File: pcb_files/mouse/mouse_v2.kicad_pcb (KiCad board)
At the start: 2 copper layers, 94.7 x 94.9 mm, 72 parts, among them J2 BT_Conn, J4 I2C_Conn, M1 Motor_DC, M2 Motor_DC, M3 CASTER_BALL, Q0 Q_Photo_NPN, Q1 Q_Photo_NPN, Q2 Q_Photo_NPN, Q3 Q_Photo_NPN, SW1 TL3315NF160Q, SW2 TL3315NF160Q, T0 Q_NMOS_DGS, T1 Q_NMOS_DGS, T2 Q_NMOS_DGS, T3 Q_NMOS_DGS, U1 Teensy3.2, U2 SN754410NE, U3 LM1084-5.0, U4 Encoder_3081, U5 Encoder_3081

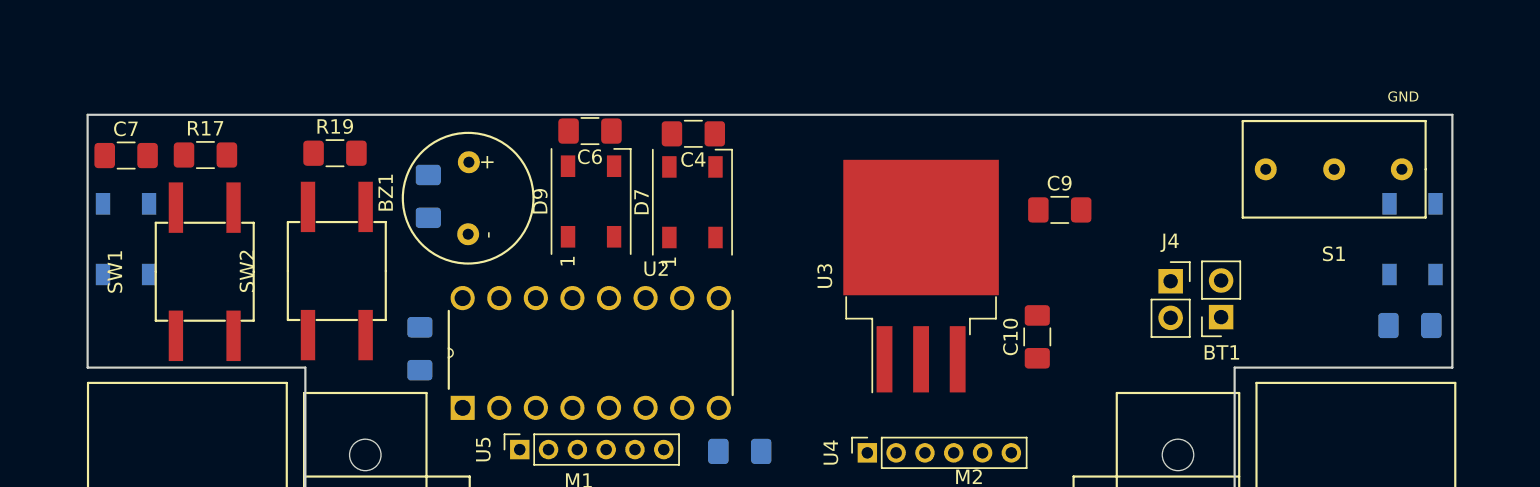
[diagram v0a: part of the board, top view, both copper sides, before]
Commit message: added usb c, rounded edges
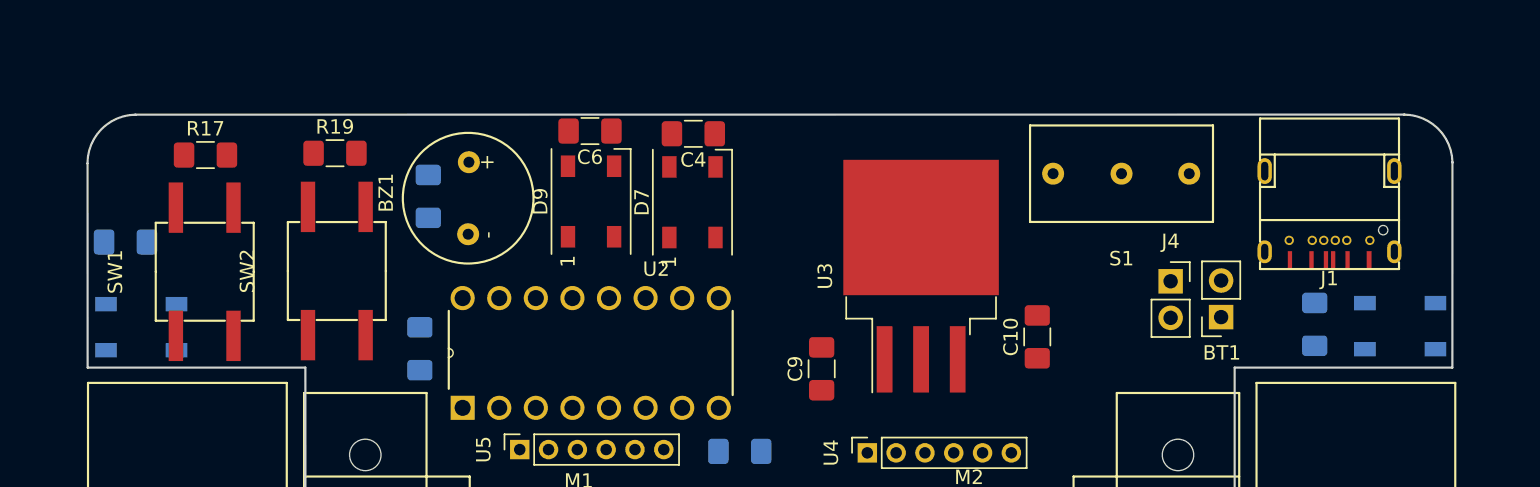
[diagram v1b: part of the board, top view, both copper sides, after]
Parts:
- added J1: USB_C_Receptacle, misc:USB_C_REDUCED_PINS, F.Cu at (198.8, 59.7)
- C7: moved to B.Cu
- moved C9 19.9 mm to (163.6, 72.3), turned to 90 degrees
- moved S1 14.8 mm to (184.4, 58.8)
- moved C5 6.61 mm to (197.8, 69.2), turned to 90 degrees
- moved D10 6.20 mm to (116.3, 69.4), turned to 180 degrees
- moved D8 6.10 mm to (203.7, 69.3), turned to 180 degrees
- moved C7 6.00 mm to (115.2, 63.5), turned to 180 degrees
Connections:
- C10 pad 1: /5v -> Net-(C10-Pad1)
- C9 pad 1: Net-(C9-Pad1) -> /vBatt
- S1 pad 1: Net-(C9-Pad1) -> Net-(C10-Pad1)
- S1 pad 2: /vBatt -> /5v
- S1 pad 3: Net-(S1-Pad3) -> /USB_VBUS
- U3 pad 2: /5v -> Net-(C10-Pad1)
- U3 pad 3: Net-(C9-Pad1) -> /vBatt
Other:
- board size 94.7 x 94.9 mm -> 94.8 x 94.9 mm
